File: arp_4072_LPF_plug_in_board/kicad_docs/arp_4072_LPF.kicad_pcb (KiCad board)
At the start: 2 copper layers, 58.4 x 50.8 mm, 80 parts, among them J1 signal_in, J2 CV_in, J3 signal_out, J4 feedback_CV_and_power, Q1 BCM857DS, Q10 MMBT3906, Q2 BCM857DS, Q3 BCM857DS, Q4 BCM857DS, Q5 BCM857DS, Q6 BCM857DS, Q7 BCM847DS135, Q8 MMBT3904, Q9 MMBT3904, U1 LM3900, U2 TL072, U3 TL072

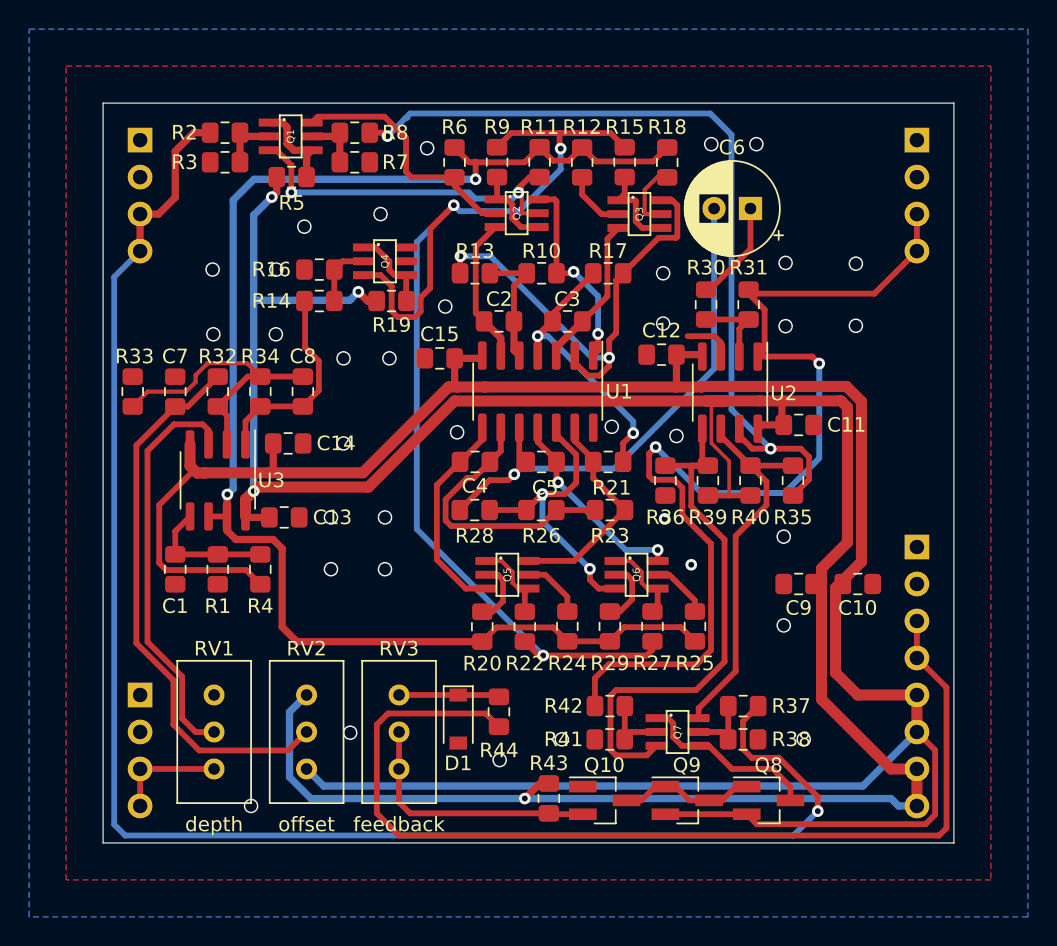
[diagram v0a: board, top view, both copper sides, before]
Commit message: fix schemo and pcb problems
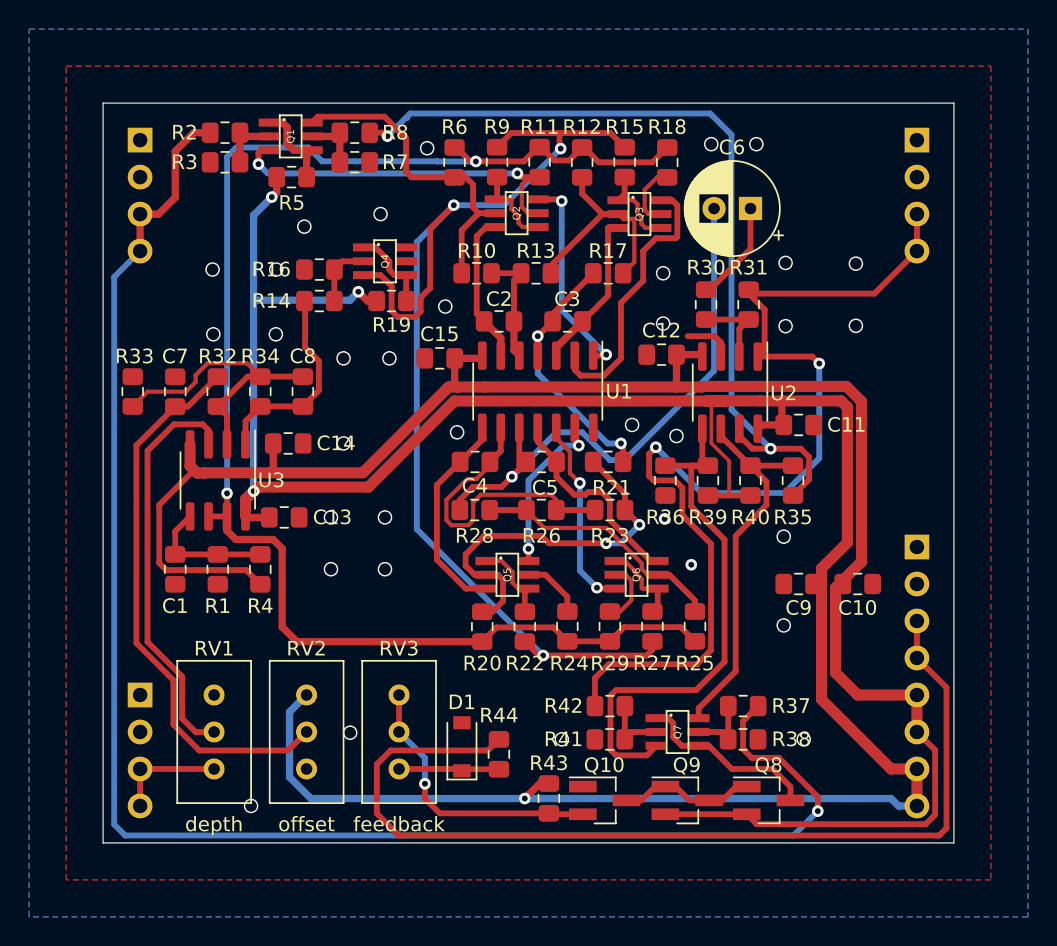
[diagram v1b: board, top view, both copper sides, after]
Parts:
- R32: value 470k -> 120k
- R8: value 15k -> 68k
- moved R10 4.46 mm to (152.6, 87.9), turned to 180 degrees
- moved R13 4.19 mm to (156.7, 87.9), turned to 180 degrees
- moved R44 2.92 mm to (154.2, 120.9), turned to 270 degrees
- moved D1 1.92 mm to (151.6, 120.4), turned to 90 degrees
- turned R11 to 90 degrees
- turned R12 to 90 degrees
- turned R18 to 90 degrees
- turned R20 to 270 degrees
- turned R24 to 270 degrees
- turned R25 to 270 degrees
- turned R29 to 270 degrees
- turned R6 to 90 degrees
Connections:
- R10 pad 2: Net-(Q2-Pad6) -> Net-(Q1-Pad6)
- R11 pad 1: /low_pass_core/v_bias -> Net-(Q1-Pad3)
- R11 pad 2: Net-(Q1-Pad3) -> /low_pass_core/v_bias
- R12 pad 1: /low_pass_core/v_bias -> Net-(Q3-Pad2)
- R12 pad 2: Net-(Q3-Pad2) -> /low_pass_core/v_bias
- R13 pad 1: Net-(Q3-Pad6) -> Net-(Q3-Pad2)
- R17 pad 2: Net-(Q3-Pad6) -> Net-(Q3-Pad2)
- R18 pad 1: /low_pass_core/v_bias -> Net-(Q3-Pad5)
- R18 pad 2: Net-(Q3-Pad5) -> /low_pass_core/v_bias
- R20 pad 1: /low_pass_core/v_bias -> Net-(Q5-Pad2)
- R20 pad 2: Net-(Q5-Pad2) -> /low_pass_core/v_bias
- R21 pad 1: Net-(Q5-Pad6) -> Net-(Q5-Pad2)
- R23 pad 2: Net-(Q5-Pad6) -> Net-(Q5-Pad2)
- R24 pad 1: /low_pass_core/v_bias -> Net-(Q5-Pad5)
- R24 pad 2: Net-(Q5-Pad5) -> /low_pass_core/v_bias
- R25 pad 1: /low_pass_core/v_bias -> Net-(Q6-Pad5)
- R25 pad 2: Net-(Q6-Pad5) -> /low_pass_core/v_bias
- R26 pad 1: Net-(Q6-Pad3) -> Net-(Q6-Pad5)
- R28 pad 2: Net-(Q6-Pad3) -> Net-(Q6-Pad5)
- R29 pad 1: /low_pass_core/v_bias -> Net-(Q6-Pad2)
- R29 pad 2: Net-(Q6-Pad2) -> /low_pass_core/v_bias
- R6 pad 1: /low_pass_core/v_bias -> Net-(Q1-Pad6)
- R6 pad 2: Net-(Q1-Pad6) -> /low_pass_core/v_bias
- RV2 pad 3: -12V -> GND
- RV3 pad 1: Net-(D1-Pad1) -> Net-(Q10-Pad2)
- RV3 pad 3: Net-(Q10-Pad2) -> Net-(D1-Pad1)
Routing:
- net -12V: track 174.4 -> 130.4 mm
- net Net-(Q5-Pad2): track 4.48 -> 25.3 mm, vias 0 -> 2
- net Net-(Q3-Pad6): track 32.7 -> 19.0 mm, vias 2 -> 0
- net Net-(Q6-Pad5): track 4.05 -> 17.7 mm
- net Net-(Q3-Pad2): track 4.23 -> 15.0 mm
- net Net-(Q6-Pad3): track 20.3 -> 13.4 mm
- net Net-(Q1-Pad6): track 17.2 -> 22.4 mm
- net Net-(Q5-Pad6): track 15.2 -> 11.3 mm, vias 0 -> 2
- net Net-(C5-Pad1): track 35.8 -> 38.8 mm
- net /feedback_VCA/feedback_CV_in: track 70.2 -> 67.5 mm
- net Net-(C4-Pad1): track 19.1 -> 21.0 mm
- net Net-(Q10-Pad2): track 17.8 -> 19.1 mm, vias 0 -> 1
- net Net-(Q4-Pad3): track 80.7 -> 79.6 mm
- net /low_pass_core/v_bias: track 100.7 -> 101.7 mm
- net Net-(C2-Pad1): track 8.69 -> 8.04 mm
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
